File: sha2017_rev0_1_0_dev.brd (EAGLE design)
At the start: 95 x 86 mm, 201 parts, among them IC1 CP210X_USB_UART, IC2 AP7215, IC3 ESP32WROOM32, IC4 MCP73833, IC5 FXL6408, IC6 CPT112, Q2 MMBT2222A, Q3 MMBT2222A, Q4 MMBT2222A, Q5 MMBT2222A, Q6 SI1304 BDL, Q7 MMBT2222A, T1 SI2301DS, T2 SI2301DS, T3 SI2301DS, X1 2908-05WB-MG, X3 JST-PH3

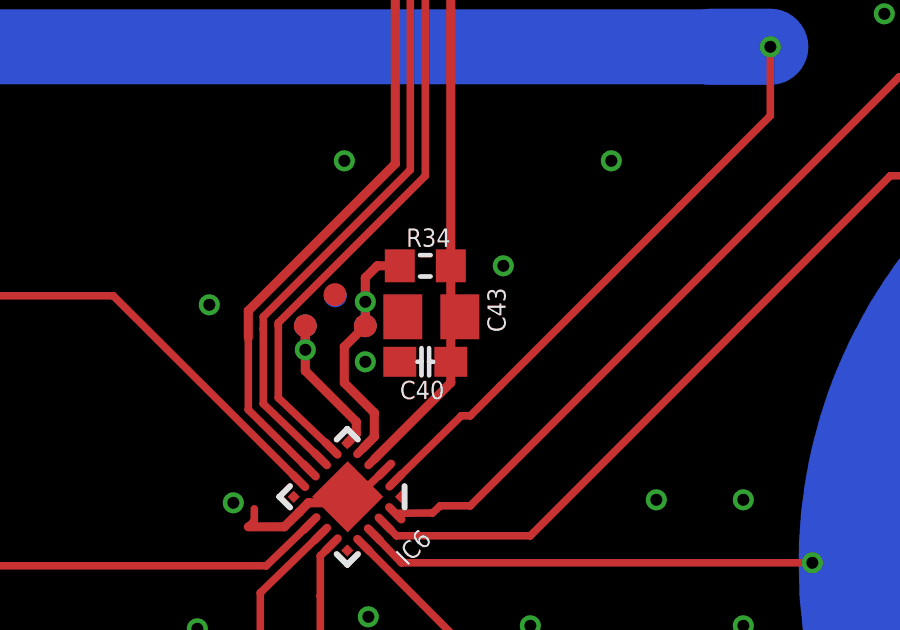
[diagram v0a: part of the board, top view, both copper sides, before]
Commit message: minor adjustments
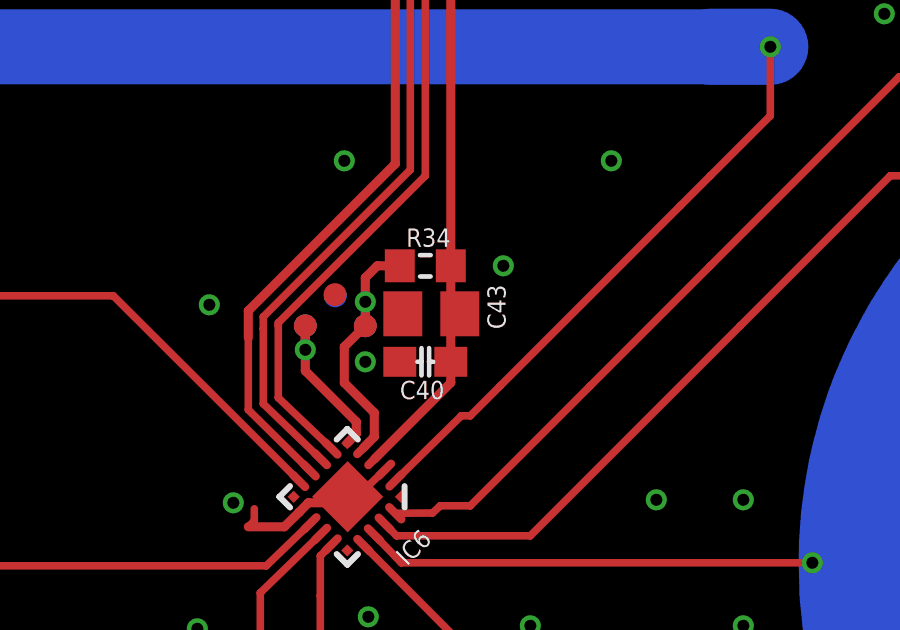
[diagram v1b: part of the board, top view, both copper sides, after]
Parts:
- moved C43 0.10 mm to (43.7, 28.4)
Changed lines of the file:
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@@
 <attribute name="VALUE" x="16.249" y="57.708" size="0.4064" layer="27" rot="R270"/>
 </element>
-<element name="C43" library="rcl" package="C0805" value="4u7/16V" x="43.7" y="28.3" smashed="yes" rot="R180">
-<attribute name="PARTNO" value="GRM21BR61C475KA88K" x="43.7" y="28.3" size="1.778" layer="27" rot="R180" display="off"/>
-<attribute name="NAME" x="45.57" y="29.27" size="0.6096" layer="25" font="vector" ratio="15" rot="R270"/>
-<attribute name="VALUE" x="44.97" y="30.84" size="1.27" layer="27" rot="R180"/>
+<element name="C43" library="rcl" package="C0805" value="4u7/16V" x="43.7" y="28.4" smashed="yes" rot="R180">
+<attribute name="PARTNO" value="GRM21BR61C475KA88K" x="43.7" y="28.4" size="1.778" layer="27" rot="R180" display="off"/>
+<attribute name="NAME" x="45.57" y="29.37" size="0.6096" layer="25" font="vector" ratio="15" rot="R270"/>
+<attribute name="VALUE" x="44.97" y="30.94" size="1.27" layer="27" rot="R180"/>
 </element>
 </elements>
@@
 <wire x1="23.25" y1="48.6" x2="23.8" y2="48.05" width="0.6096" layer="1"/>
 <contactref element="C43" pad="1"/>
-<wire x1="44.65" y1="28.3" x2="44.408578125" y2="28.2" width="0.3048" layer="1" curve="-45"/>
+<wire x1="44.65" y1="28.4" x2="44.408578125" y2="28.2" width="0.3048" layer="1" curve="-45"/>
 <wire x1="44.408578125" y1="28.2" x2="44.35" y2="28.2" width="0.3048" layer="1"/>
 </signal>
